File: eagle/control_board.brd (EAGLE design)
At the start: 160 x 100 mm, 24 parts, among them Q1 TIP122V

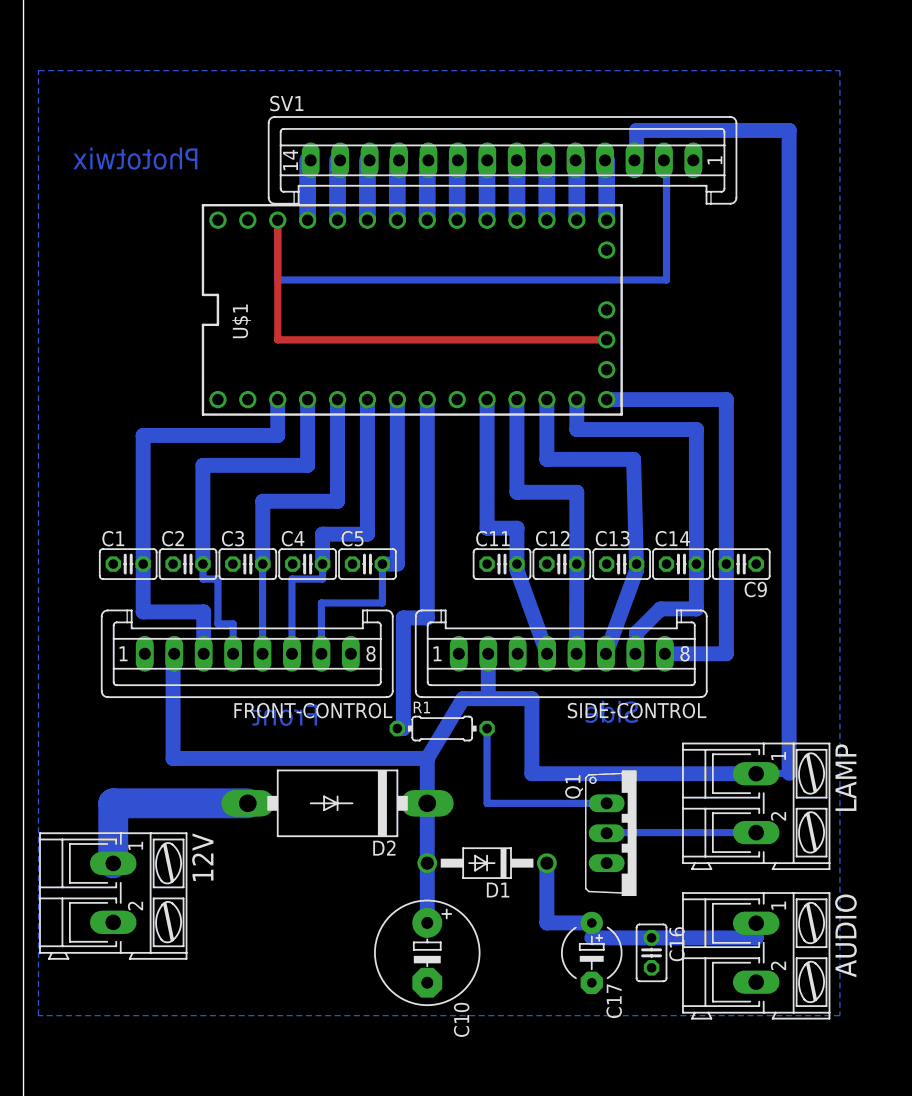
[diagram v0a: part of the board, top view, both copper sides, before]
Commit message: Autocad plan
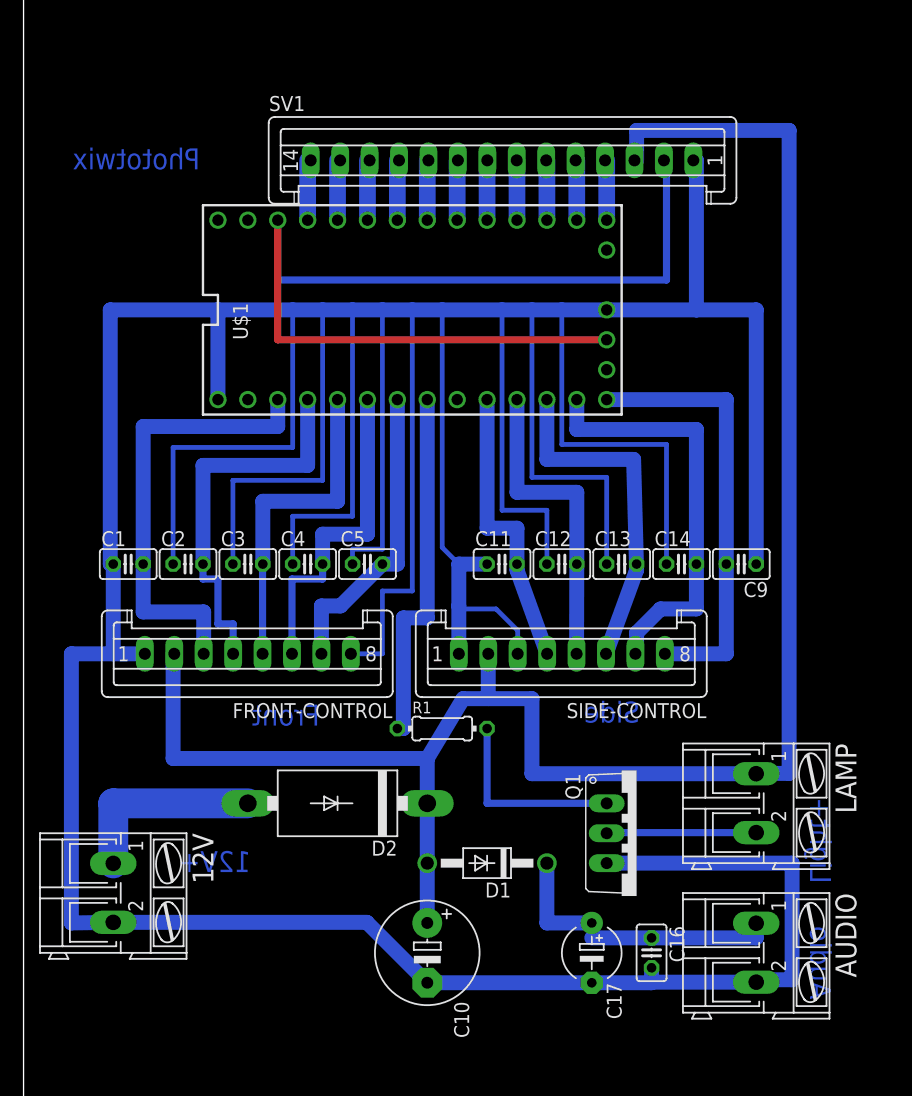
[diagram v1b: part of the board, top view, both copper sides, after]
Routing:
- net GND: track 0.00 -> 516.1 mm
- net BTN_GALLERY: track 28.0 -> 26.2 mm
- removed copper zone on layer 16, net GND
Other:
- board text added: "12V+"
- board text added: "Audio"
- board text added: "Light+"
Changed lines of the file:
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@@
 <layer number="19" name="Unrouted" color="6" fill="1" visible="yes" active="yes"/>
 <layer number="20" name="Dimension" color="15" fill="1" visible="no" active="yes"/>
-<layer number="21" name="tPlace" color="7" fill="1" visible="yes" active="yes"/>
+<layer number="21" name="tPlace" color="7" fill="1" visible="no" active="yes"/>
 <layer number="22" name="bPlace" color="7" fill="1" visible="no" active="yes"/>
-<layer number="23" name="tOrigins" color="15" fill="1" visible="yes" active="yes"/>
+<layer number="23" name="tOrigins" color="15" fill="1" visible="no" active="yes"/>
 <layer number="24" name="bOrigins" color="15" fill="1" visible="no" active="yes"/>
 <layer number="25" name="tNames" color="7" fill="1" visible="no" active="yes"/>
@@
 <text x="25.146" y="35.814" size="1.778" layer="16" rot="MR0">Front</text>
 <text x="52.324" y="36.068" size="1.778" layer="16" rot="MR0">Side</text>
+<text x="19.304" y="23.368" size="1.778" layer="16" rot="MR0">12V+</text>
+<text x="68.58" y="18.796" size="1.778" layer="16" rot="MR270">Audio</text>
+<text x="68.58" y="29.718" size="1.778" layer="16" rot="MR270">Light+</text>
 </plain>
 <attributes>
@@
 <contactref element="SV1" pad="1"/>
 <contactref element="SIDE-CONTROL" pad="3"/>
-<polygon width="0.6096" layer="16">
-<vertex x="1.27" y="91.44"/>
-<vertex x="69.342" y="91.44"/>
-<vertex x="69.342" y="11.176"/>
-<vertex x="1.27" y="11.176"/>
-</polygon>
+<wire x1="56.89" y1="83.82" x2="57.15" y2="83.82" width="1.27" layer="16"/>
+<wire x1="57.15" y1="83.82" x2="57.15" y2="71.12" width="1.27" layer="16"/>
+<wire x1="57.15" y1="71.12" x2="49.53" y2="71.12" width="1.27" layer="16"/>
+<wire x1="49.53" y1="71.12" x2="45.72" y2="71.12" width="1.27" layer="16"/>
+<wire x1="45.72" y1="71.12" x2="43.18" y2="71.12" width="1.27" layer="16"/>
+<wire x1="43.18" y1="71.12" x2="40.64" y2="71.12" width="1.27" layer="16"/>
+<wire x1="40.64" y1="71.12" x2="35.56" y2="71.12" width="1.27" layer="16"/>
+<wire x1="35.56" y1="71.12" x2="33.02" y2="71.12" width="1.27" layer="16"/>
+<wire x1="33.02" y1="71.12" x2="30.48" y2="71.12" width="1.27" layer="16"/>
+<wire x1="30.48" y1="71.12" x2="27.94" y2="71.12" width="1.27" layer="16"/>
+<wire x1="27.94" y1="71.12" x2="25.4" y2="71.12" width="1.27" layer="16"/>
+<wire x1="25.4" y1="71.12" x2="22.86" y2="71.12" width="1.27" layer="16"/>
+<wire x1="22.86" y1="71.12" x2="16.51" y2="71.12" width="1.27" layer="16"/>
+<wire x1="16.51" y1="71.12" x2="16.51" y2="63.5" width="1.27" layer="16"/>
+<wire x1="7.62" y1="49.53" x2="7.366" y2="49.53" width="1.27" layer="16"/>
+<wire x1="7.366" y1="49.53" x2="7.366" y2="71.12" width="1.27" layer="16"/>
+<wire x1="7.366" y1="71.12" x2="16.51" y2="71.12" width="1.27" layer="16"/>
+<wire x1="62.23" y1="49.53" x2="62.23" y2="71.12" width="1.27" layer="16"/>
+<wire x1="62.23" y1="71.12" x2="57.15" y2="71.12" width="1.27" layer="16"/>
+<wire x1="34.29" y1="13.97" x2="48.26" y2="13.97" width="1.27" layer="16"/>
+<wire x1="48.26" y1="13.97" x2="53.34" y2="13.97" width="1.27" layer="16"/>
+<wire x1="53.34" y1="14.0208" x2="53.34" y2="15.24" width="1.27" layer="16"/>
+<wire x1="62.23" y1="14.0208" x2="53.34" y2="14.0208" width="1.27" layer="16"/>
+<wire x1="53.34" y1="14.0208" x2="53.34" y2="13.97" width="1.27" layer="16"/>
+<wire x1="39.37" y1="49.53" x2="36.97" y2="49.53" width="1.27" layer="16"/>
+<wire x1="36.97" y1="49.53" x2="36.97" y2="45.974" width="1.27" layer="16"/>
+<wire x1="36.97" y1="45.974" x2="36.97" y2="41.91" width="1.27" layer="16"/>
+<wire x1="49.53" y1="24.13" x2="65.278" y2="24.13" width="1.27" layer="16"/>
+<wire x1="65.278" y1="24.13" x2="65.278" y2="14.224" width="1.27" layer="16"/>
+<wire x1="65.278" y1="14.224" x2="62.23" y2="14.224" width="1.27" layer="16"/>
+<wire x1="62.23" y1="14.224" x2="62.23" y2="14.0208" width="1.27" layer="16"/>
+<wire x1="10.3" y1="41.91" x2="7.62" y2="41.91" width="1.27" layer="16"/>
+<wire x1="7.62" y1="41.91" x2="7.62" y2="49.53" width="1.27" layer="16"/>
+<wire x1="12.7" y1="49.53" x2="12.7" y2="59.436" width="0.4064" layer="16"/>
+<wire x1="12.7" y1="59.436" x2="22.86" y2="59.436" width="0.4064" layer="16"/>
+<wire x1="22.86" y1="59.436" x2="22.86" y2="71.12" width="0.4064" layer="16"/>
+<wire x1="17.78" y1="49.53" x2="17.78" y2="56.642" width="0.4064" layer="16"/>
+<wire x1="17.78" y1="56.642" x2="25.4" y2="56.642" width="0.4064" layer="16"/>
+<wire x1="25.4" y1="56.642" x2="25.4" y2="71.12" width="0.4064" layer="16"/>
+<wire x1="22.86" y1="49.53" x2="22.86" y2="53.594" width="0.4064" layer="16"/>
+<wire x1="22.86" y1="53.594" x2="27.94" y2="53.594" width="0.4064" layer="16"/>
+<wire x1="27.94" y1="53.594" x2="27.94" y2="71.12" width="0.4064" layer="16"/>
+<wire x1="27.94" y1="49.53" x2="27.94" y2="50.8" width="0.4064" layer="16"/>
+<wire x1="27.94" y1="50.8" x2="30.48" y2="50.8" width="0.4064" layer="16"/>
+<wire x1="30.48" y1="50.8" x2="30.48" y2="71.12" width="0.4064" layer="16"/>
+<wire x1="27.8" y1="41.91" x2="30.48" y2="41.91" width="0.4064" layer="16"/>
+<wire x1="30.48" y1="41.91" x2="30.48" y2="47.244" width="0.4064" layer="16"/>
+<wire x1="30.48" y1="47.244" x2="33.02" y2="47.244" width="0.4064" layer="16"/>
+<wire x1="33.02" y1="47.244" x2="33.02" y2="71.12" width="0.4064" layer="16"/>
+<wire x1="36.97" y1="49.53" x2="35.56" y2="50.94" width="0.4064" layer="16"/>
+<wire x1="35.56" y1="50.94" x2="35.56" y2="71.12" width="0.4064" layer="16"/>
+<wire x1="41.97" y1="41.91" x2="41.97" y2="43.882" width="0.4064" layer="16"/>
+<wire x1="41.97" y1="43.882" x2="40.132" y2="45.72" width="0.4064" layer="16"/>
+<wire x1="40.132" y1="45.72" x2="37.224" y2="45.72" width="0.4064" layer="16"/>
+<wire x1="37.224" y1="45.72" x2="36.97" y2="45.974" width="0.4064" layer="16"/>
+<wire x1="44.45" y1="49.53" x2="44.45" y2="54.102" width="0.4064" layer="16"/>
+<wire x1="44.45" y1="54.102" x2="40.64" y2="54.102" width="0.4064" layer="16"/>
+<wire x1="40.64" y1="54.102" x2="40.64" y2="71.12" width="0.4064" layer="16"/>
+<wire x1="49.53" y1="49.53" x2="49.53" y2="56.896" width="0.4064" layer="16"/>
+<wire x1="49.53" y1="56.896" x2="43.18" y2="56.896" width="0.4064" layer="16"/>
+<wire x1="43.18" y1="56.896" x2="43.18" y2="71.12" width="0.4064" layer="16"/>
+<wire x1="54.61" y1="49.53" x2="54.61" y2="59.69" width="0.4064" layer="16"/>
+<wire x1="54.61" y1="59.69" x2="45.72" y2="59.69" width="0.4064" layer="16"/>
+<wire x1="45.72" y1="59.69" x2="45.72" y2="71.12" width="0.4064" layer="16"/>
+<wire x1="7.62" y1="19.1008" x2="4.064" y2="19.05" width="1.27" layer="16"/>
+<wire x1="4.064" y1="19.05" x2="4.064" y2="41.91" width="1.27" layer="16"/>
+<wire x1="4.064" y1="41.91" x2="7.62" y2="41.91" width="1.27" layer="16"/>
+<wire x1="34.29" y1="13.97" x2="29.1592" y2="19.1008" width="1.27" layer="16"/>
+<wire x1="29.1592" y1="19.1008" x2="7.62" y2="19.1008" width="1.27" layer="16"/>
 </signal>
 <signal name="BTN_PHOTO">
@@
 <contactref element="C1" pad="2"/>
 <contactref element="U$1" pad="1"/>
-<wire x1="21.59" y1="63.5" x2="21.59" y2="60.452" width="1.27" layer="16"/>
-<wire x1="21.59" y1="60.452" x2="10.16" y2="60.452" width="1.27" layer="16"/>
-<wire x1="10.16" y1="60.452" x2="10.16" y2="49.53" width="1.27" layer="16"/>
+<wire x1="21.59" y1="63.5" x2="21.59" y2="61.214" width="1.27" layer="16"/>
+<wire x1="21.59" y1="61.214" x2="10.16" y2="61.214" width="1.27" layer="16"/>
+<wire x1="10.16" y1="61.214" x2="10.16" y2="49.53" width="1.27" layer="16"/>
 <wire x1="10.16" y1="49.53" x2="10.16" y2="45.466" width="1.27" layer="16"/>
 <wire x1="10.16" y1="45.466" x2="15.3" y2="45.466" width="1.27" layer="16"/>
@@
 <contactref element="FRONT-CONTROL" pad="7"/>
 <contactref element="C5" pad="2"/>
-<wire x1="30.48" y1="49.53" x2="30.48" y2="46.228" width="0.6096" layer="16"/>
-<wire x1="30.48" y1="46.228" x2="25.3" y2="46.228" width="0.6096" layer="16"/>
-<wire x1="25.3" y1="46.228" x2="25.3" y2="41.91" width="0.6096" layer="16"/>
+<wire x1="25.3" y1="46.228" x2="25.3" y2="45.974" width="0.6096" layer="16"/>
 <contactref element="U$1" pad="5"/>
+<wire x1="25.3" y1="45.974" x2="25.3" y2="41.91" width="1.27" layer="16"/>
 <wire x1="31.75" y1="63.5" x2="31.75" y2="49.53" width="1.27" layer="16"/>
 <wire x1="31.75" y1="49.53" x2="30.48" y2="49.53" width="1.27" layer="16"/>
+<wire x1="30.48" y1="49.53" x2="26.924" y2="45.974" width="1.27" layer="16"/>
+<wire x1="26.924" y1="45.974" x2="25.3" y2="45.974" width="1.27" layer="16"/>
 </signal>
 <signal name="BTN_PRINT">
@@
 <wire x1="52.07" y1="86.36" x2="65.024" y2="86.36" width="1.27" layer="16"/>
 <wire x1="65.024" y1="86.36" x2="65.024" y2="31.75" width="1.27" layer="16"/>
-<wire x1="65.024" y1="31.75" x2="62.23" y2="31.75" width="0.6096" layer="16"/>
+<wire x1="65.024" y1="31.75" x2="62.23" y2="31.75" width="1.27" layer="16"/>
 <wire x1="62.23" y1="31.75" x2="62.23" y2="31.7246" width="0.6096" layer="16"/>
 </signal>
